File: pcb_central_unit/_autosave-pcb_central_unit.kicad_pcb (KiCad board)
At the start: 2 copper layers, 120.8 x 64.5 mm, 16 parts, among them J1 CMD_PAN, J2 GLASS_0, J3 GLASS_1, J4 STEPPER_0, J5 STEPPER_1, J6 DCDC_BOOSTER, J7 ALIM_5V, J8 SPARE_GPIO_0, J9 SPARE_GPIO_1, U1 TMC2208_SILENTSTEPSTICK-TMC22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, U2 TMC2208_SILENTSTEPSTICK-TMC22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, U3 ESP32_DevKit_V1_DOIT_30_pin

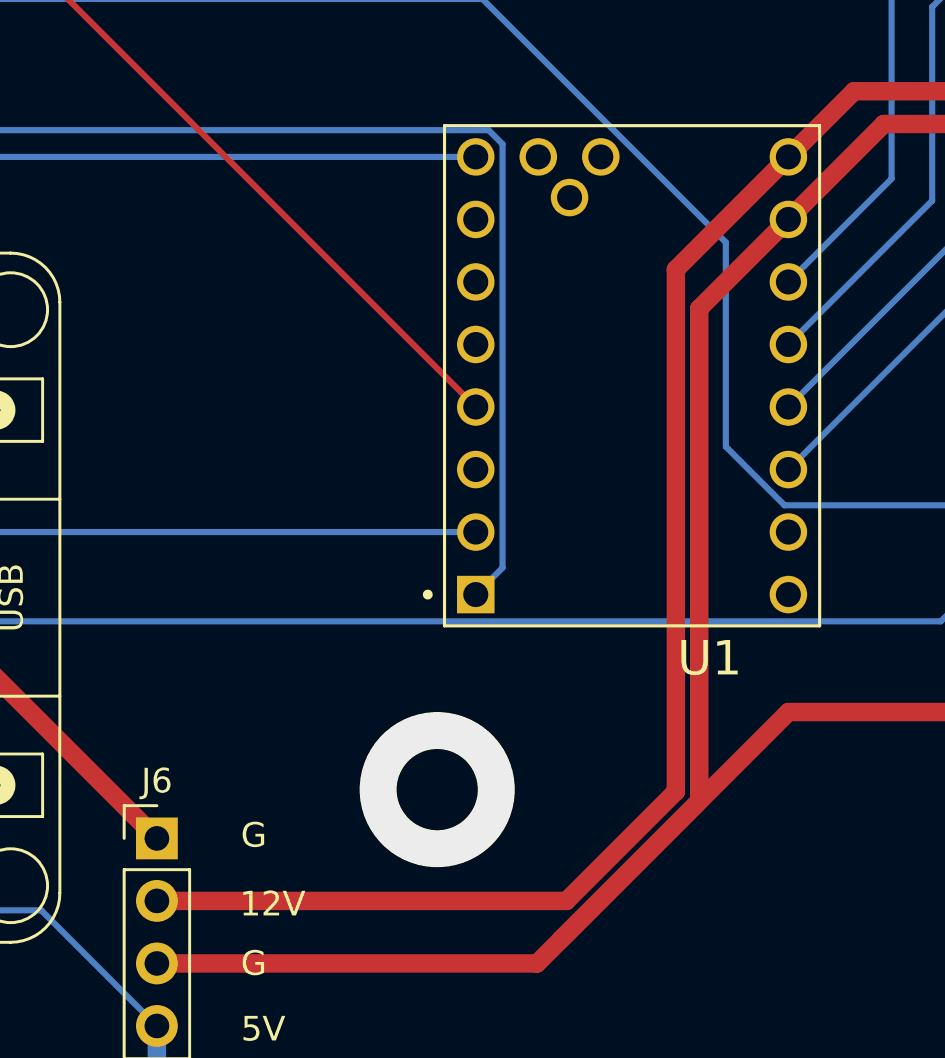
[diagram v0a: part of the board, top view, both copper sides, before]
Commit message: PCB v2.5
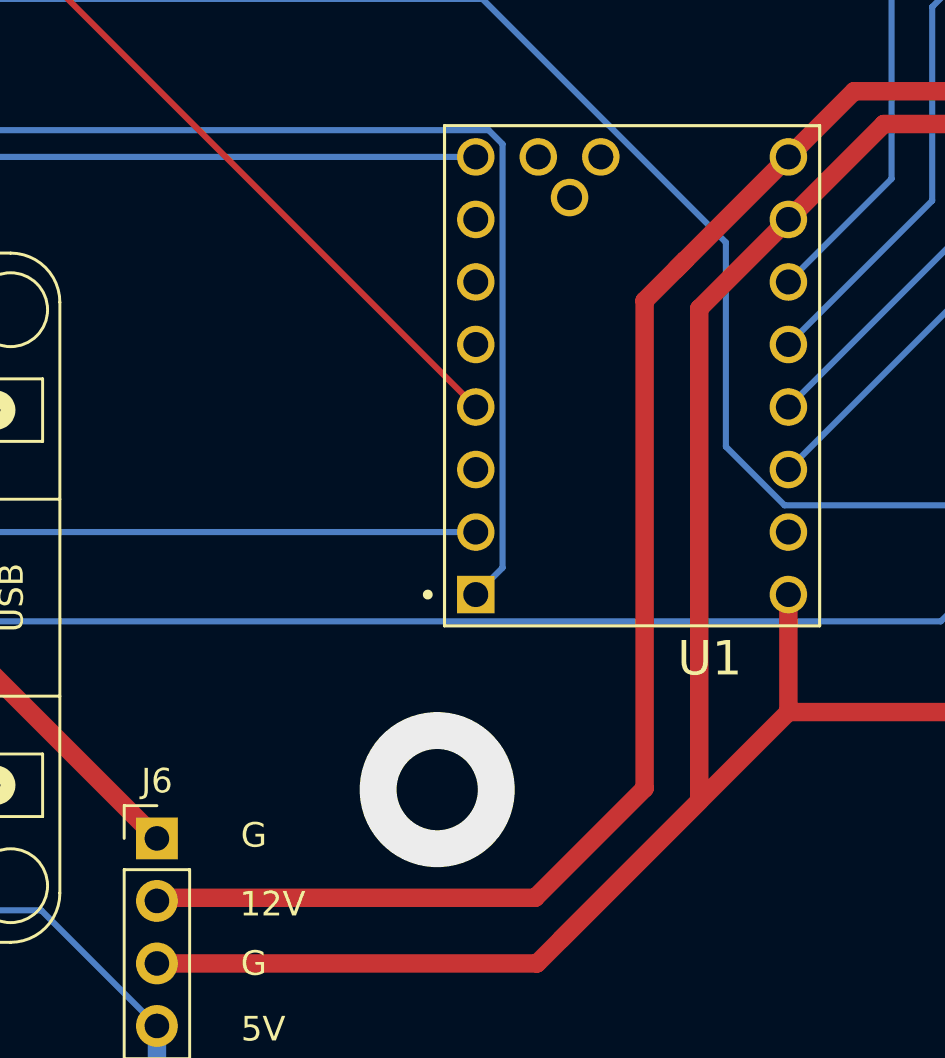
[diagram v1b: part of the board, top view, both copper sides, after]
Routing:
- net GND: track 234.8 -> 239.6 mm
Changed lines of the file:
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@@
     (thickness 1.6)
     (drawings 12)
-    (tracks 203)
+    (tracks 207)
     (zones 0)
     (modules 16)
@@
   (segment (start 151.818484 97.482516) (end 132.461 97.482516) (width 0.75) (layer F.Cu) (net 1))
   (segment (start 156.591 92.71) (end 151.818484 97.482516) (width 0.75) (layer F.Cu) (net 1))
+  (segment (start 132.461 92.71) (end 132.461 97.482516) (width 0.75) (layer F.Cu) (net 1))
   (segment (start 101.727 122.809) (end 102.235 122.301) (width 0.25) (layer B.Cu) (net 2))
   (segment (start 53.351598 64.16099) (end 49.243999 68.268589) (width 0.25) (layer B.Cu) (net 2))
@@
   (segment (start 135.128 72.263) (end 132.461 74.93) (width 0.75) (layer F.Cu) (net 7))
   (segment (start 155.829 72.263) (end 135.128 72.263) (width 0.75) (layer F.Cu) (net 7))
-  (segment (start 123.444 105.156) (end 106.807 105.156) (width 0.75) (layer F.Cu) (net 7))
-  (segment (start 127.889 79.502) (end 127.889 100.711) (width 0.75) (layer F.Cu) (net 7))
-  (segment (start 127.889 100.711) (end 123.444 105.156) (width 0.75) (layer F.Cu) (net 7))
-  (segment (start 132.461 74.93) (end 127.889 79.502) (width 0.75) (layer F.Cu) (net 7))
+  (segment (start 126.619 100.584) (end 122.174 105.029) (width 0.75) (layer F.Cu) (net 7))
+  (segment (start 126.619 80.772) (end 128.27 79.121) (width 0.75) (layer F.Cu) (net 7))
+  (segment (start 126.619 100.584) (end 126.619 80.772) (width 0.75) (layer F.Cu) (net 7))
+  (segment (start 128.27 79.121) (end 127.889 79.502) (width 0.75) (layer F.Cu) (net 7))
+  (segment (start 132.461 74.93) (end 128.27 79.121) (width 0.75) (layer F.Cu) (net 7))
+  (segment (start 106.934 105.029) (end 106.807 105.156) (width 0.75) (layer F.Cu) (net 7))
+  (segment (start 122.174 105.029) (end 106.934 105.029) (width 0.75) (layer F.Cu) (net 7))
   (segment (start 86.646001 121.444001) (end 85.471 120.269) (width 0.25) (layer B.Cu) (net 10))
   (segment (start 88.575001 121.444001) (end 86.646001 121.444001) (width 0.25) (layer B.Cu) (net 10))
@@
   (segment (start 81.915 75.946) (end 77.724 80.137) (width 0.25) (layer B.Cu) (net 53))
   (segment (start 81.915 71.12) (end 81.915 75.946) (width 0.25) (layer B.Cu) (net 53))
-  (zone (net 1) (net_name GND) (layer B.Cu) (hatch edge 0.508)
+  (zone (net 24) (net_name +3.3V) (layer F.Cu) (hatch edge 0.508)
     (connect_pads (clearance 0.508))
     (min_thickness 0.254)
@@
     )
   )
-  (zone (net 24) (net_name +3.3V) (layer F.Cu) (hatch edge 0.508)
+  (zone (net 1) (net_name GND) (layer B.Cu) (hatch edge 0.508)
     (connect_pads (clearance 0.508))
     (min_thickness 0.254)
